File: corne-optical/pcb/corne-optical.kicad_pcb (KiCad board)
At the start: 2 copper layers, 145.7 x 94.9 mm, 77 parts, among them J1 MJ-4PP-9, J2 OLED, J3 LED, J4 Conn_01x02, J5 Conn_01x02, P1 i2c-pin, P2 i2c-pin, SW1 SW_PUSH, SW10 SW_PUSH, SW11 SW_PUSH, SW12 SW_PUSH, SW13 SW_PUSH, SW14 SW_PUSH, SW15 SW_PUSH, SW16 SW_PUSH, SW17 SW_PUSH, SW18 SW_PUSH, SW19 SW_PUSH, SW2 SW_PUSH, SW20 SW_PUSH, SW21 SW_PUSH, SW3 SW_PUSH, SW4 SW_PUSH, SW5 SW_PUSH, SW6 SW_PUSH, SW7 SW_PUSH, SW8 SW_PUSH, SW9 SW_PUSH, U1 ProMicro

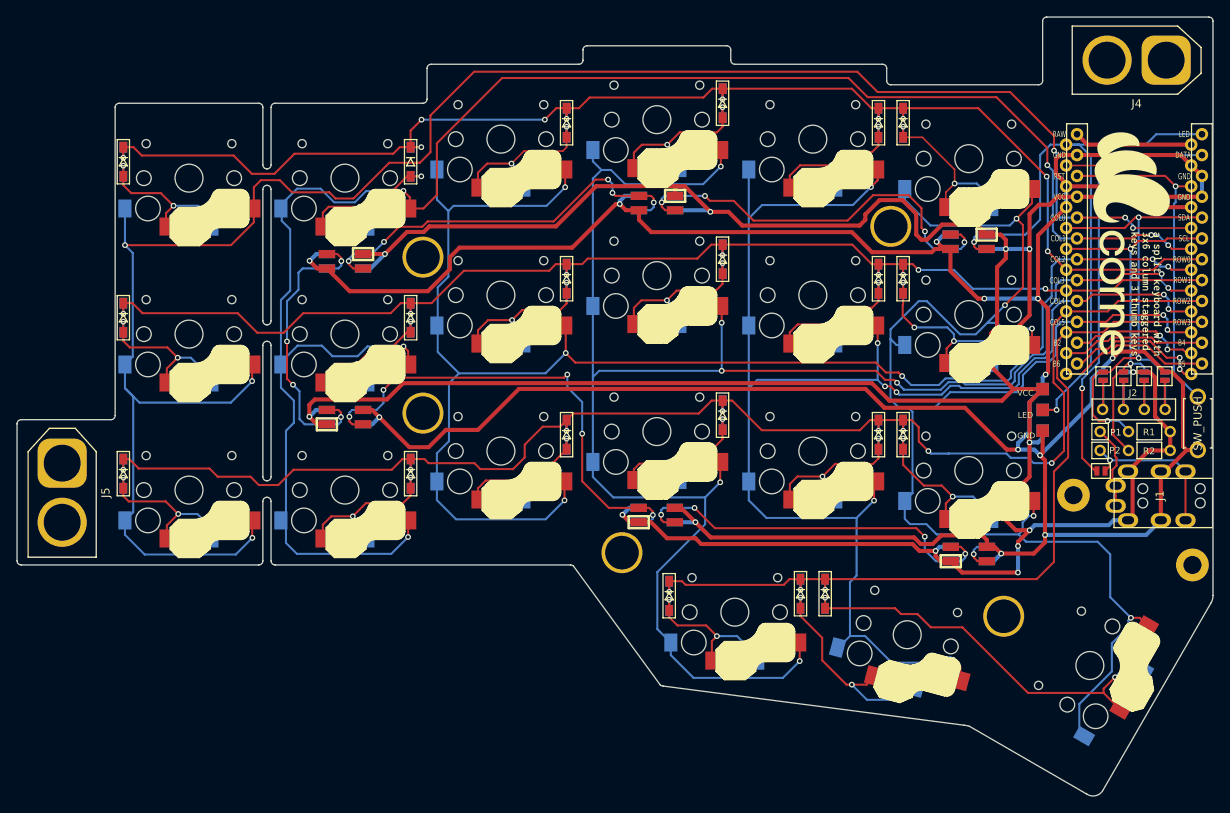
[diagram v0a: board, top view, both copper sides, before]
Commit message: Trying to workout phantom copper
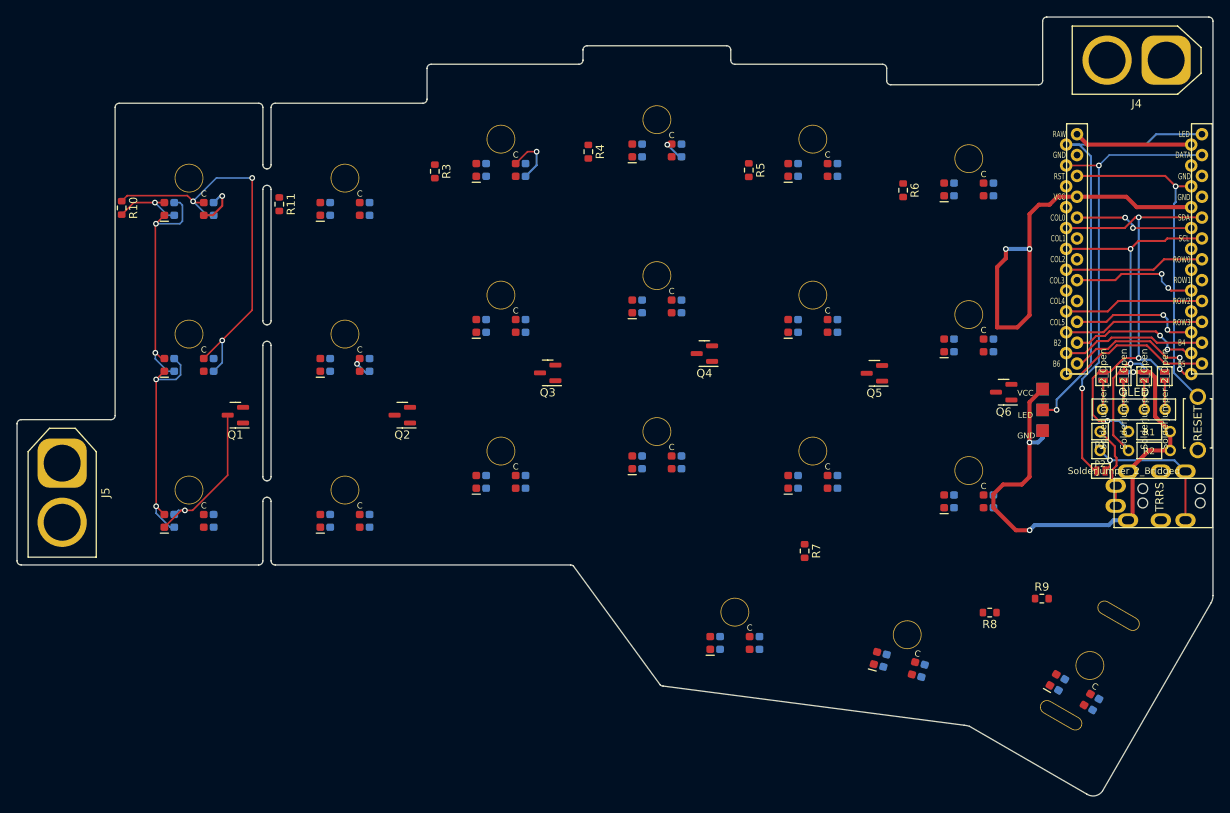
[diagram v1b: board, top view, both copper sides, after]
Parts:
- removed ? (x7): , kbd:LEGO_HOLE
- removed D1, D10, D11, D12, D13, D14, D15, D16, D17, D18, D19, D2, D20, D21, D3, D4, D5, D6, D7, D8, D9: D, kbd:D3_SMD
- removed G*** (x2): LOGO, kbd:corne
- removed L22, L23, L24, L25, L26, L27: SK6812MINI, kbd:SK6812MINI_underglow_rev
- added Q1: Q_NMOS_GSD, Package_TO_SOT_SMD:SOT-23, F.Cu at (75.7, 106.0)
- added Q2: Q_NMOS_GSD, Package_TO_SOT_SMD:SOT-23, F.Cu at (96.0, 106.0)
- added Q3: Q_NMOS_GSD, Package_TO_SOT_SMD:SOT-23, F.Cu at (113.7, 100.8)
- added Q4: Q_NMOS_GSD, Package_TO_SOT_SMD:SOT-23, F.Cu at (132.8, 98.5)
- added Q5: Q_NMOS_GSD, Package_TO_SOT_SMD:SOT-23, F.Cu at (153.5, 100.9)
- added Q6: Q_NMOS_GSD, Package_TO_SOT_SMD:SOT-23, F.Cu at (169.2, 103.2)
- added R10: 70R, Resistor_SMD:R_0603_1608Metric, F.Cu at (61.8, 80.8)
- added R11: 70R, Resistor_SMD:R_0603_1608Metric, F.Cu at (81.0, 80.3)
- added R3: 70R, Resistor_SMD:R_0603_1608Metric, F.Cu at (100.0, 76.3)
- added R4: 70R, Resistor_SMD:R_0603_1608Metric, F.Cu at (118.7, 73.9)
- added R5: 70R, Resistor_SMD:R_0603_1608Metric, F.Cu at (138.2, 76.2)
- added R6: 70R, Resistor_SMD:R_0603_1608Metric, F.Cu at (157.0, 78.6)
- added R7: 190R, Resistor_SMD:R_0603_1608Metric, F.Cu at (145.0, 122.5)
- added R8: 190R, Resistor_SMD:R_0603_1608Metric, F.Cu at (167.6, 130.1)
- added R9: 190R, Resistor_SMD:R_0603_1608Metric, F.Cu at (173.9, 128.3)
- J2: value OLED -> Conn_01x04
- J3: value LED -> Conn_01x03
- JP1: value (none) -> SolderJumper_2_Bridged
- JP2, JP3, JP4, JP5, JP6, JP7, JP8, JP9: value (none) -> SolderJumper_2_Open
- P1, P2: value i2c-pin -> Conn_01x01
- RSW1: value SW_PUSH -> SW_Push
- SW1, SW10, SW11, SW12, SW13, SW14, SW15, SW16, SW17, SW18, SW19, SW2, SW20, SW3, SW4, SW5, SW6, SW7, SW8, SW9: value SW_PUSH -> Keychron_LP_Optical; footprint kbd:Choc_Hotswap -> optical:Keychron_LP_Optical
- SW21: value SW_PUSH -> Keychron_LP_Optical; footprint kbd:Choc_Hotswap_1.5u -> optical:Keychron_LP_Optical_1.5u
- turned SW1 to 0 degrees
- turned SW10 to 0 degrees
- turned SW11 to 0 degrees
- turned SW12 to 0 degrees
- turned SW13 to 0 degrees
- turned SW14 to 0 degrees
- turned SW15 to 0 degrees
- turned SW16 to 0 degrees
- turned SW17 to 0 degrees
- turned SW18 to 0 degrees
- turned SW19 to 0 degrees
- turned SW2 to 0 degrees
- turned SW20 to -15 degrees
- turned SW21 to -30 degrees
- turned SW3 to 0 degrees
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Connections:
- SW1 pad 1: col0 -> Net-(R10-Pad2)
- SW1 pad 2: Net-(D1-Pad2) -> Net-(SW1-Pad2)
- SW10 pad 1: col3 -> Net-(SW10-Pad1)
- SW10 pad 2: Net-(D10-Pad2) -> Net-(SW10-Pad2)
- SW11 pad 1: col4 -> Net-(SW11-Pad1)
- SW11 pad 2: Net-(D11-Pad2) -> Net-(SW11-Pad2)
- SW12 pad 1: col5 -> Net-(SW12-Pad1)
- SW12 pad 2: Net-(D12-Pad2) -> Net-(SW12-Pad2)
- SW13 pad 1: col0 -> Net-(SW13-Pad1)
- SW13 pad 2: Net-(D13-Pad2) -> /col0_sink
- SW14 pad 1: col1 -> Net-(SW14-Pad1)
- SW14 pad 2: Net-(D14-Pad2) -> /col1_sink
- SW15 pad 1: col2 -> Net-(SW15-Pad1)
- SW15 pad 2: Net-(D15-Pad2) -> unconnected-(SW15-Pad2)
- SW16 pad 1: col3 -> Net-(SW10-Pad2)
- SW16 pad 2: Net-(D16-Pad2) -> /col3_sink
- SW17 pad 1: col4 -> Net-(SW11-Pad2)
- SW17 pad 2: Net-(D17-Pad2) -> /col4_sink
- SW18 pad 1: col5 -> Net-(SW12-Pad2)
- SW18 pad 2: Net-(D18-Pad2) -> /col5_sink
- SW19 pad 1: col3 -> Net-(R7-Pad2)
- SW19 pad 2: Net-(D19-Pad2) -> /col3_sink
- SW2 pad 1: col1 -> Net-(R11-Pad2)
- SW2 pad 2: Net-(D2-Pad2) -> Net-(SW2-Pad2)
- SW20 pad 1: col4 -> Net-(R8-Pad2)
- SW20 pad 2: Net-(D20-Pad2) -> /col4_sink
- SW21 pad 1: col5 -> Net-(R9-Pad2)
- SW21 pad 2: Net-(D21-Pad2) -> /col5_sink
- SW3 pad 1: col2 -> Net-(R3-Pad2)
- SW3 pad 2: Net-(D3-Pad2) -> Net-(SW3-Pad2)
- SW4 pad 1: col3 -> Net-(R4-Pad2)
- SW4 pad 2: Net-(D4-Pad2) -> Net-(SW10-Pad1)
- SW5 pad 1: col4 -> Net-(R5-Pad2)
- SW5 pad 2: Net-(D5-Pad2) -> Net-(SW11-Pad1)
- SW6 pad 1: col5 -> Net-(R6-Pad2)
- SW6 pad 2: Net-(D6-Pad2) -> Net-(SW12-Pad1)
- SW7 pad 1: col0 -> Net-(SW1-Pad2)
- SW7 pad 2: Net-(D7-Pad2) -> Net-(SW13-Pad1)
- SW8 pad 1: col1 -> Net-(SW2-Pad2)
- SW8 pad 2: Net-(D8-Pad2) -> Net-(SW14-Pad1)
- SW9 pad 1: col2 -> Net-(SW3-Pad2)
- SW9 pad 2: Net-(D9-Pad2) -> Net-(SW15-Pad1)
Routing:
- net GND: track 412.9 -> 0.00 mm, vias 13 -> 0
- net col0: track 239.4 -> 14.7 mm, vias 6 -> 2
- net col1: track 220.3 -> 0.00 mm, vias 6 -> 0
- net VCC: track 389.0 -> 176.6 mm, vias 12 -> 11
- net col3: track 214.9 -> 15.6 mm, vias 8 -> 2
- net col2: track 188.6 -> 0.00 mm, vias 6 -> 0
- net col4: track 184.7 -> 0.00 mm, vias 8 -> 0
- net col5: track 191.4 -> 15.9 mm, vias 7 -> 2
- net row2: track 178.7 -> 17.1 mm, vias 8 -> 0
- net row1: track 155.8 -> 0.00 mm, vias 8 -> 0
- net row0: track 168.8 -> 22.4 mm, vias 10 -> 1
- net row3: track 102.8 -> 17.1 mm, vias 3 -> 0
- net Net-(L25-Pad1): track 58.9 -> 0.00 mm, vias 5 -> 0
- net Net-(L23-Pad3): track 50.0 -> 0.00 mm, vias 4 -> 0
- net Net-(D21-Pad2): track 49.9 -> 0.00 mm, vias 2 -> 0
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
